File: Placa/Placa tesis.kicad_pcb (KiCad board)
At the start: 2 copper layers, 100 x 50 mm, 110 parts, among them J1 Conn_01x03, J10 Conn_01x01, J11 USB_B_Micro, J12 Conn_01x01, J13 Conn_01x05, J14 Conn_01x08, J15 Conn_01x04, J2 Conn_01x04, J3 Conn_01x02, J4 Conn_01x03, J5 Conn_01x04, J6 Conn_01x08, J7 Conn_01x11, J8 Conn_01x11, J9 Conn_01x03, Q1 Q_NMOS_GDS, Q2 Q_NMOS_GDS, Q3 Q_NMOS_GDS, Q4 Q_NMOS_GDS, SW1 SW_Push, SW2 SW_Push, U2 Nodemcuv_3, U3 INA226, U4 LM3464AMH_NOPB, U5 ESP-12E, U6 ESP-12E, U9 FT230XS

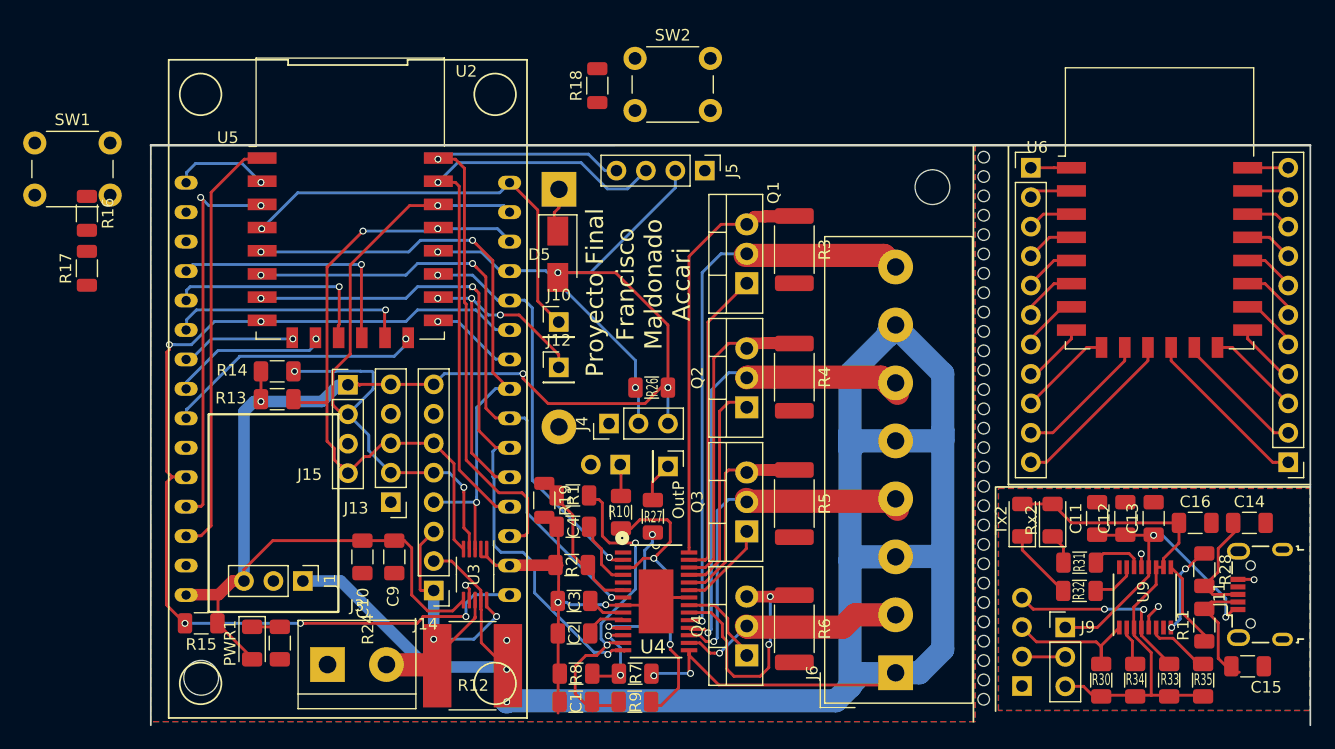
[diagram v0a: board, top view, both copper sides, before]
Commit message: La venganza
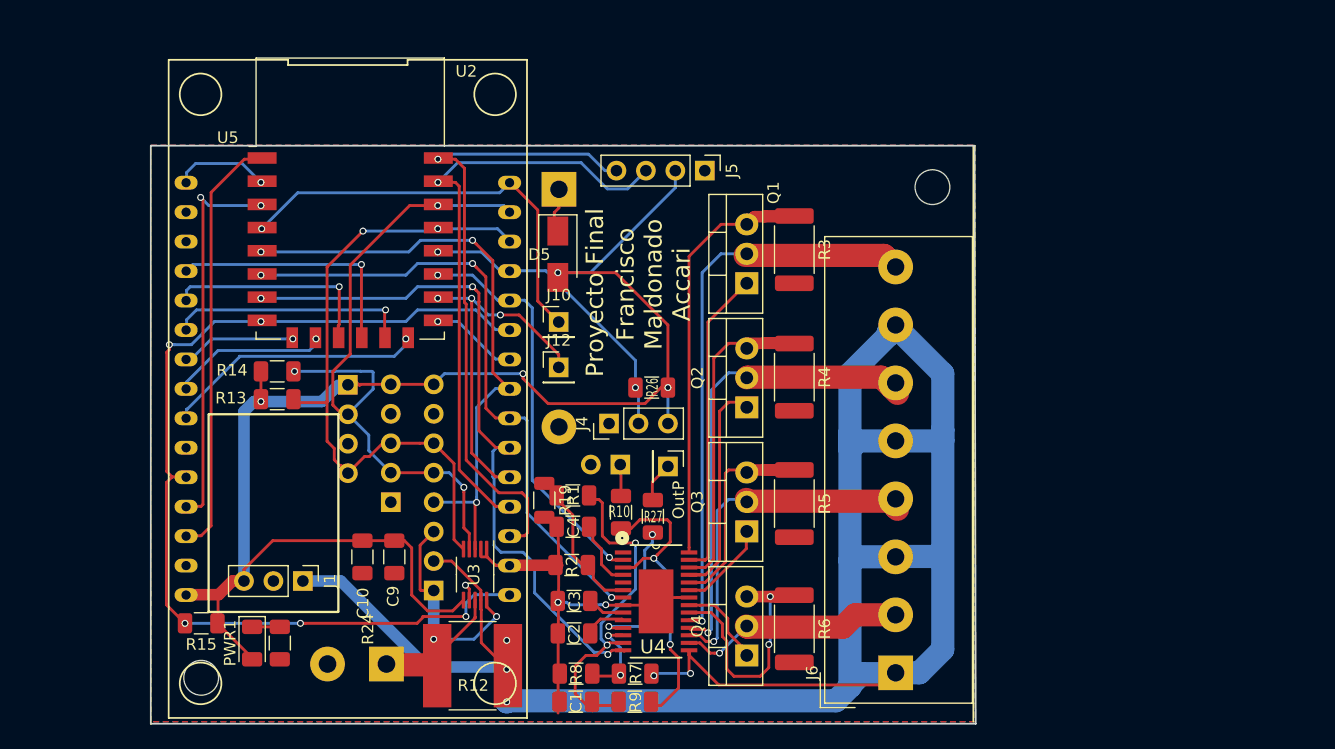
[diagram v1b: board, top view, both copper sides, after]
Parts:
- removed C11: 4.7u, Capacitor_SMD:C_1206_3216Metric
- removed C12, C16: 100n, Capacitor_SMD:C_1206_3216Metric
- removed C13: 10n, Capacitor_SMD:C_1206_3216Metric
- removed C14, C15: 47p, Capacitor_SMD:C_1206_3216Metric
- removed J11: USB_B_Micro, Connector_USB:USB_Micro-B_Wuerth_629105150521
- removed J2: Conn_01x04, Connector_PinHeader_2.54mm:PinHeader_1x04_P2.54mm_Vertical
- removed J7, J8: Conn_01x11, Connector_PinHeader_2.54mm:PinHeader_1x11_P2.54mm_Vertical
- removed J9: Conn_01x03, Connector_PinHeader_2.54mm:PinHeader_1x03_P2.54mm_Vertical
- removed R11, R28: 27, Resistor_SMD:R_1206_3216Metric
- removed R16, R17, R18: 10k, Resistor_SMD:R_1206_3216Metric
- removed R30, R33, R34, R35: 10K, Resistor_SMD:R_1206_3216Metric
- removed R31, R32: 270, Resistor_SMD:R_1206_3216Metric
- removed the REF** at (155.3, 91.2)
- removed the REF** at (155.3, 76.1)
- removed the REF** at (155.3, 74.5)
- removed the REF** at (155.3, 72.8)
- removed the REF** at (155.3, 71.1)
- removed the REF** at (155.3, 67.8)
- removed the REF** at (155.3, 69.5)
- removed the REF** at (155.3, 66.1)
- removed the REF** at (155.3, 64.5)
- removed the REF** at (155.3, 62.8)
- removed the REF** at (155.3, 61.1)
- removed the REF** at (155.3, 89.5)
- removed the REF** at (155.3, 59.4)
- removed the REF** at (155.3, 57.8)
- removed the REF** at (155.3, 56.1)
- removed the REF** at (155.3, 54.4)
- removed the REF** at (155.3, 52.8)
- removed the REF** at (155.3, 51.1)
- removed the REF** at (155.3, 49.4)
- removed the REF** at (155.3, 47.8)
- removed the REF** at (155.3, 46.1)
- removed the REF** at (155.3, 44.4)
- removed the REF** at (155.3, 87.8)
- removed the REF** at (155.3, 86.2)
- removed the REF** at (155.3, 84.5)
- removed the REF** at (155.3, 82.8)
- removed the REF** at (155.3, 81.1)
- removed the REF** at (155.3, 79.5)
- removed the REF** at (155.3, 77.8)
- removed Rx2, Tx2: LED, LED_SMD:LED_1206_3216Metric
- removed SW1, SW2: SW_Push, Button_Switch_THT:SW_PUSH_6mm
- removed U6: ESP-12E, RF_Module:ESP-12E
- removed U9: FT230XS, Package_SO:SSOP-16_3.9x4.9mm_P0.635mm
- J1: value Conn_01x03 -> OKI-78SR
- J13: value Conn_01x05 -> BH1750; moved to B.Cu
- J14: value Conn_01x08 -> INA226; moved to B.Cu
- J15: moved to B.Cu
- J3: value Conn_01x02 -> FUENTE; moved to B.Cu
- J4: value Conn_01x03 -> DHT11
- J5: value Conn_01x04 -> COMM
- moved J3 5.08 mm to (103.1, 86.1), turned to 180 degrees
- turned J13 to 0 degrees
- turned J14 to 0 degrees
- turned J15 to 180 degrees
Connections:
- J3 pad 1: GND -> VinS
- J3 pad 2: VinS -> GND
- R15 pad 2: Net-(R15-Pad2) -> V5
- U2 pad 11: Net-(R15-Pad2) -> V5
- U2 pad 16: Net-(R15-Pad2) -> V5
- U2 pad 25: Net-(R15-Pad2) -> V5
- U5 pad 8: Net-(R15-Pad2) -> V5
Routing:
- net Net-(R15-Pad2): track 88.5 -> 0.00 mm, vias 5 -> 0
- net V5: track 129.5 -> 218.1 mm, vias 4 -> 9
- net Net-(C16-Pad1): track 43.4 -> 0.00 mm
- net Net-(C11-Pad1): track 29.0 -> 0.00 mm, vias 2 -> 0
- net Net-(J2-Pad4): track 16.7 -> 0.00 mm, vias 2 -> 0
- net Net-(J8-Pad1): track 14.9 -> 0.00 mm
- net Net-(J7-Pad11): track 14.9 -> 0.00 mm
- net Net-(J2-Pad3): track 12.8 -> 0.00 mm
- net Net-(J7-Pad10): track 11.8 -> 0.00 mm
- net Net-(J8-Pad2): track 11.4 -> 0.00 mm
- net Net-(C14-Pad1): track 10.3 -> 0.00 mm
- net Net-(C15-Pad1): track 10.2 -> 0.00 mm
- net Net-(J8-Pad3): track 8.10 -> 0.00 mm
- net Net-(J7-Pad9): track 8.10 -> 0.00 mm
- net Net-(R28-Pad1): track 7.73 -> 0.00 mm, vias 2 -> 0
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- removed copper zone on B.Cu, net GND2
- removed copper zone on F.Cu, net GND2
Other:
- board size 100 x 50 mm -> 71.1 x 49.9 mm
